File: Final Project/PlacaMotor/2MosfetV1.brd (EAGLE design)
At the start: 55.9 x 39.6 mm, 23 parts, among them IC1 ATTINY44-SSU

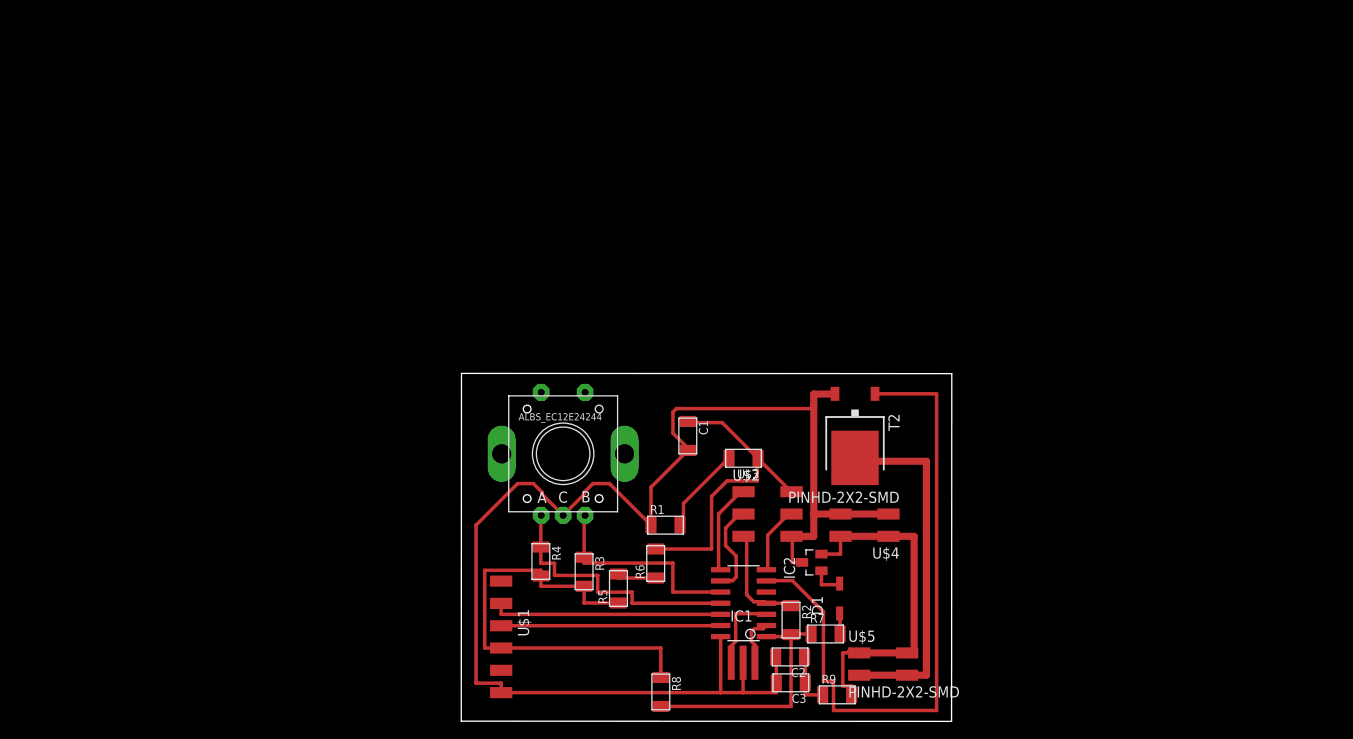
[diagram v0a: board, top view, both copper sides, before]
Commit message: lala
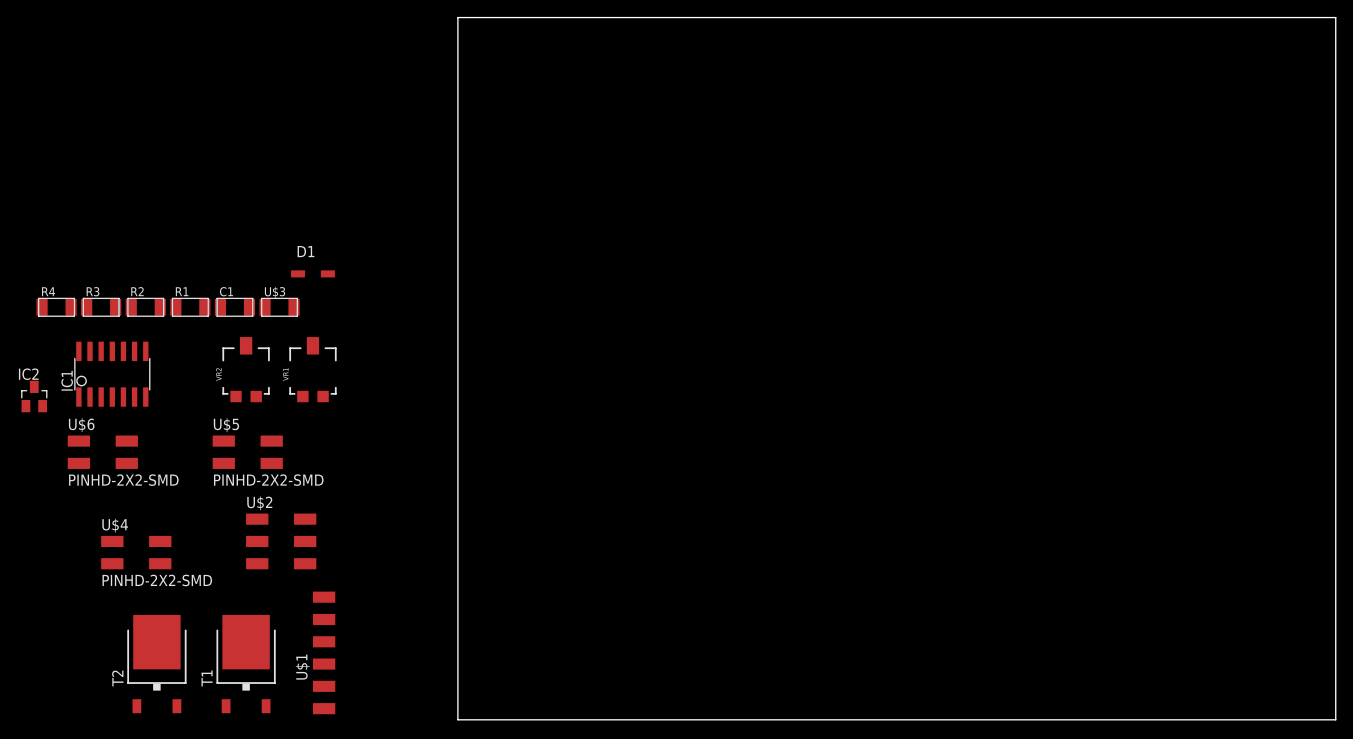
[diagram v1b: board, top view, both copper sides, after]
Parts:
- removed C2: 10uF, fab:C1206FAB
- removed C3: 0.1uF, fab:C1206FAB
- removed R5, R6, R7, R8, R9: 0, fab:R1206FAB
- removed U$7: RESONATOR, fab:EFOBM
- added T1: (no value), fab:TO252
- added VR1, VR2: 5k, SparkFun-Resistors:TRIMPOT-SMD-5MM
- R3, R4: value 10k -> 0
- U$6: value ALBS_ENCODER_STEC12E08 -> PINHD-2X2-SMD; device Rotary Encoder:STEC12E08 -> fab:2X02SMD
- moved IC2 90.6 mm to (-48.3, 36.8), turned to 0 degrees
- moved T2 83.7 mm to (-34.3, 6.35), turned to 0 degrees
- moved U$4 83.4 mm to (-36.8, 19.1), turned to 0 degrees
- moved R2 81.7 mm to (-35.6, 47.0), turned to 0 degrees
- moved IC1 76.5 mm to (-39.4, 39.4), turned to 0 degrees
- moved U$5 76.3 mm to (-24.1, 30.5)
- moved D1 70.5 mm to (-16.5, 50.8), turned to 0 degrees
- moved R3 62.7 mm to (-40.6, 47.0), turned to 0 degrees
- moved R4 62.3 mm to (-45.7, 47.0), turned to 0 degrees
- moved R1 59.5 mm to (-30.5, 47.0)
- moved U$3 55.6 mm to (-20.3, 47.0), turned to 0 degrees
- moved U$2 55.5 mm to (-20.3, 20.3)
- moved C1 53.6 mm to (-25.4, 47.0), turned to 0 degrees
- moved U$6 52.6 mm to (-40.6, 30.5)
- moved U$1 20.3 mm to (-15.2, 7.62), turned to 0 degrees
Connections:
- removed net CRYSTAL2: IC1.2, U$7.3
- removed net ENC1: IC1.10, R3.1, U$6.P$B
- removed net ENC2: IC1.11, R4.1, U$6.P$A
- removed net N$5: IC1.5
- new net AIRPUMP: IC1.5, T1.1
- new net ANALOG: IC1.11, VR1.B
- new net ANALOG2: IC1.10, VR2.B
- new net MOSFET2: T1.3, U$6.3, U$6.4
- new net N$7: IC1.2
- net 0: now also T1.2, VR1.C, VR2.C; no longer C2.2, C3.2, U$6.P$C, U$7.2
- net 12V: now also U$6.1, U$6.2; no longer C2.1, C3.1, R9.1, R9.2
- net CRYSTAL1: no longer U$7.1
- net VCC: now also R3.1, R4.1, VR1.A, VR2.A; no longer R5.1, R5.2, R6.1, R6.2, R7.1, R7.2, R8.1, R8.2
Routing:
- net 0: track 160.3 -> 0.00 mm
- net VCC: track 123.1 -> 0.00 mm
- net MOTOR: track 75.2 -> 0.00 mm
- net 12V: track 47.7 -> 0.00 mm
- net MOSFET: track 40.5 -> 0.00 mm
- net ENC2: track 30.5 -> 0.00 mm
- net RX: track 26.3 -> 0.00 mm
- net TX: track 25.1 -> 0.00 mm
- net ENC1: track 24.4 -> 0.00 mm
- net RST: track 12.6 -> 0.00 mm
- net SCK: track 10.9 -> 0.00 mm
- net MISO: track 10.9 -> 0.00 mm
- net N$1: track 10.1 -> 0.00 mm
- net CRYSTAL1: track 9.33 -> 0.00 mm
- net MOSI: track 7.86 -> 0.00 mm
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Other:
- board size 55.9 x 39.6 mm -> 100 x 80 mm
